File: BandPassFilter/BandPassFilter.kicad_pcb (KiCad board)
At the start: 2 copper layers, 98 x 84 mm, 72 parts, among them J1 OUT, J10 OUT, J11 INP, J12 OUT, J13 Conn_Coaxial, J14 INP, J15 OUT, J16 Conn_Coaxial, J2 INP, J3 INP, J4 OUT, J5 INP, J6 OUT, J7 INP, J8 OUT, J9 INP

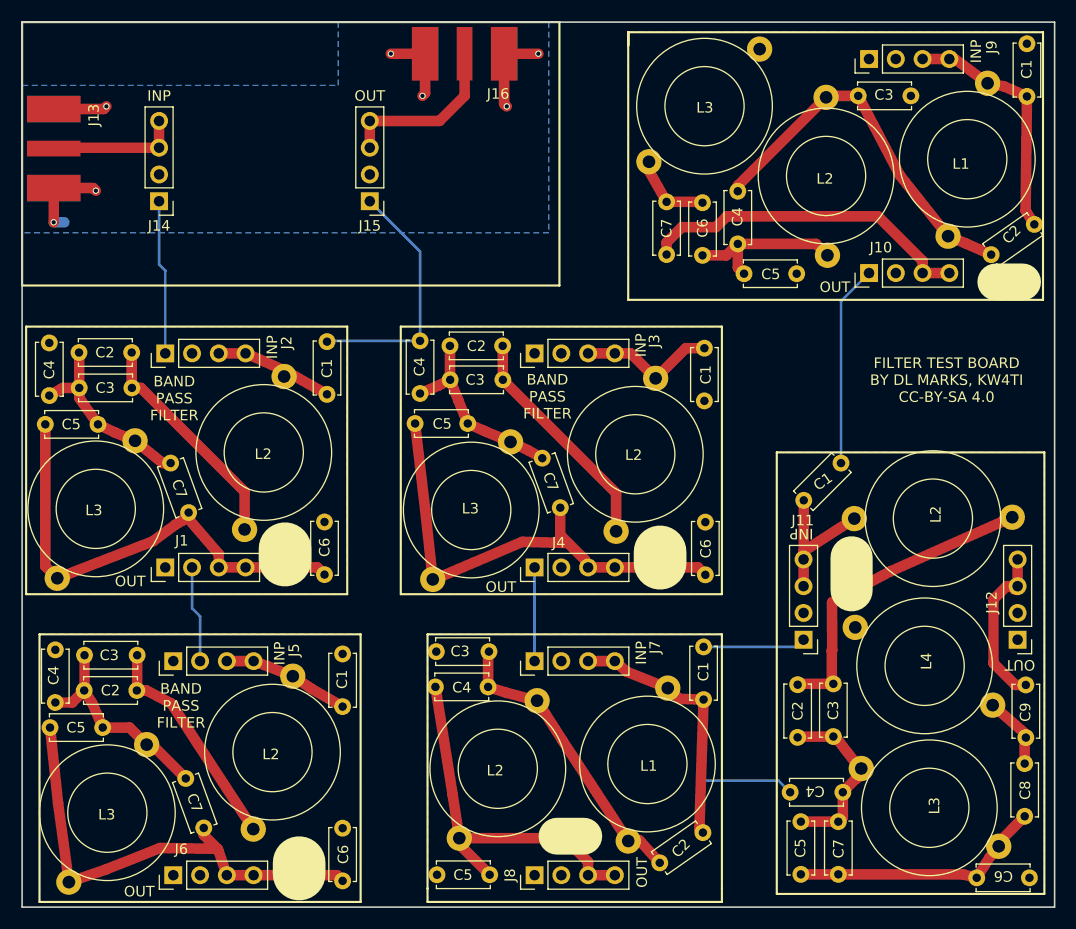
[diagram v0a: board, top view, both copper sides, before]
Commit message: Made capacitors on board dual footprint
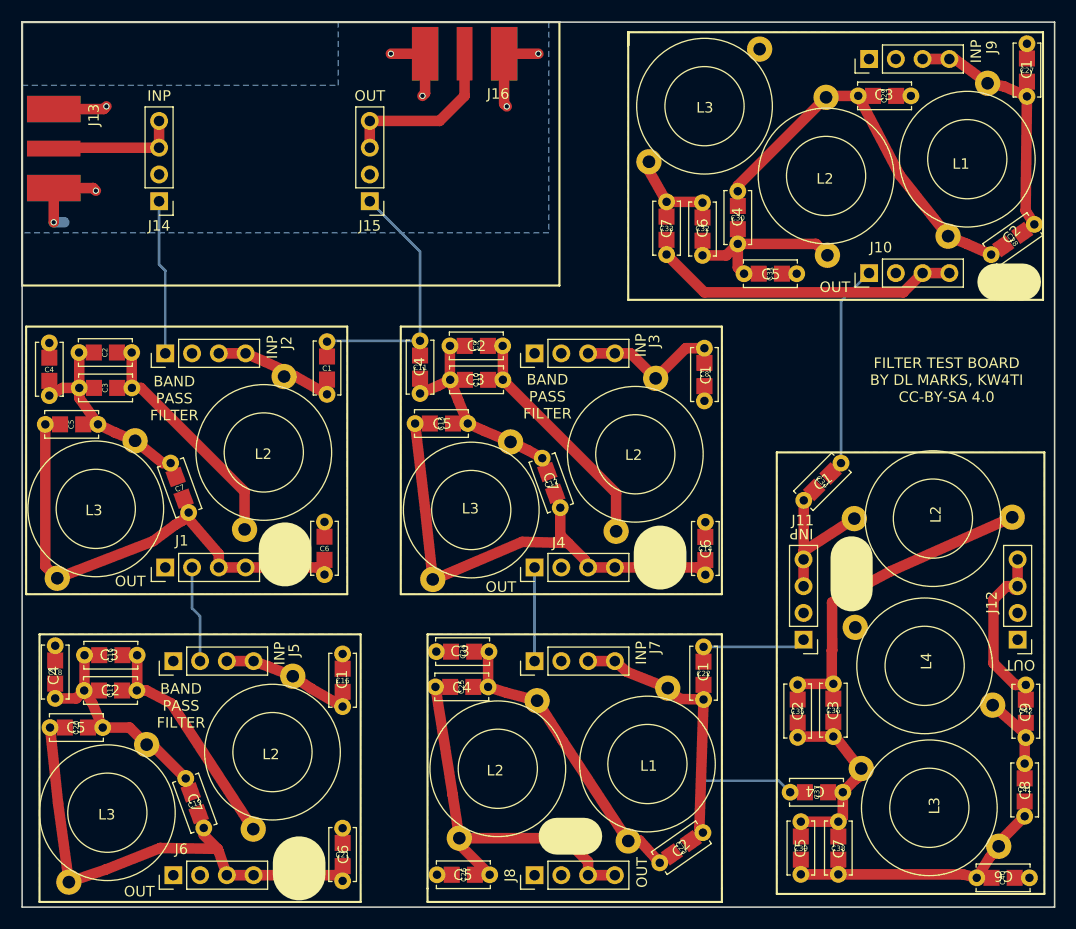
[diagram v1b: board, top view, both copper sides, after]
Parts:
- C1, C10, C11, C12, C13, C14, C15, C16, C17, C18, C19, C2, C20, C21, C22, C23, C24, C25, C26, C27, C28, C29, C3, C30, C31, C32, C33, C34, C35, C36, C37, C38, C39, C4, C40, C41, C42, C5, C6, C7, C8, C9: footprint Capacitors_THT:C_Disc_D5.0mm_W2.5mm_P5.00mm -> BandPassFilter:C_Disc_D5.0mm_W2.5mm_P5.00mm_Dual
- moved C18 0.39 mm to (122.1, 119.2)
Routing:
- net Net-(C33-Pad2): track 31.9 -> 30.2 mm
